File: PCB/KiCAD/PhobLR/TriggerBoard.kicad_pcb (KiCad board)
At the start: 2 copper layers, 9.7 x 41.7 mm, 5 parts, among them J1 L, J2 R, SW1 L, SW2 R

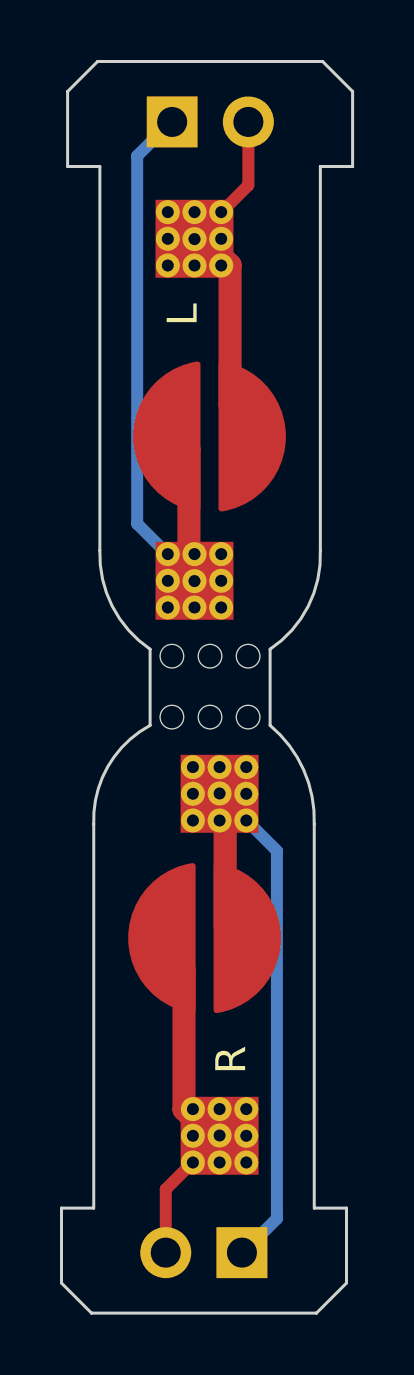
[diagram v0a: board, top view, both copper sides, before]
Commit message: Update TriggerBoard.kicad_pcb
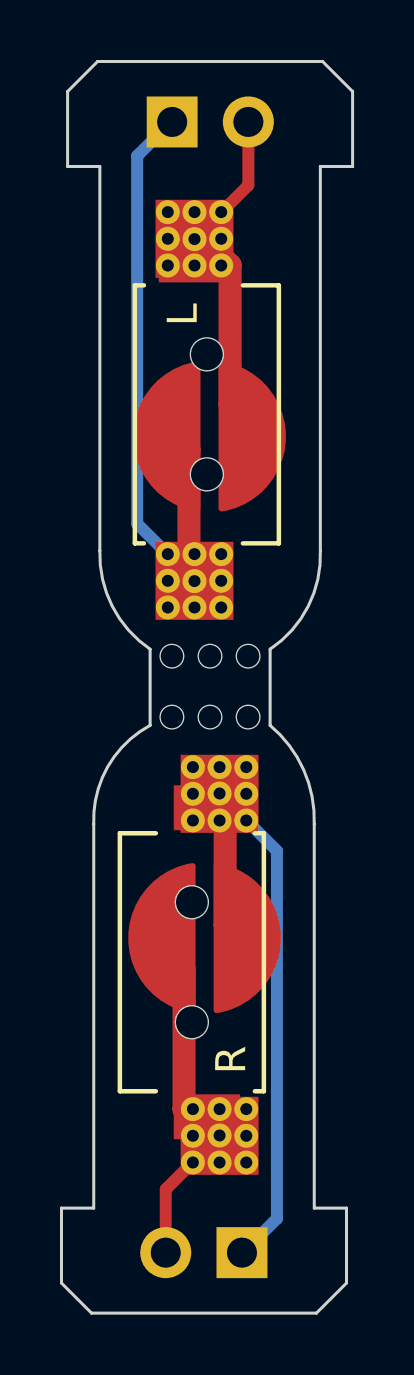
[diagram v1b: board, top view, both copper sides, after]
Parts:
- added ?: , clipboard:b50812ef-01b3-4199-b131-0dd827ad1ccd, F.Cu at (111.0, 68.3)
- added ?: , clipboard:b50812ef-01b3-4199-b131-0dd827ad1ccd, F.Cu at (105.5, 74.8)
